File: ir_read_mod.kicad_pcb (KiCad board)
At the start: 2 copper layers, 42 x 42 mm, 25 parts, among them J1 Conn_01x04_Female, J2 Conn_01x05_Female, J3 Conn_01x01_Female, J4 Conn_01x02_Female, Q1 Q_Photo_NPN, SW1 SW_Coded_SH-7070, SW2 SW_SPDT, U1 PIC16F1503-IP

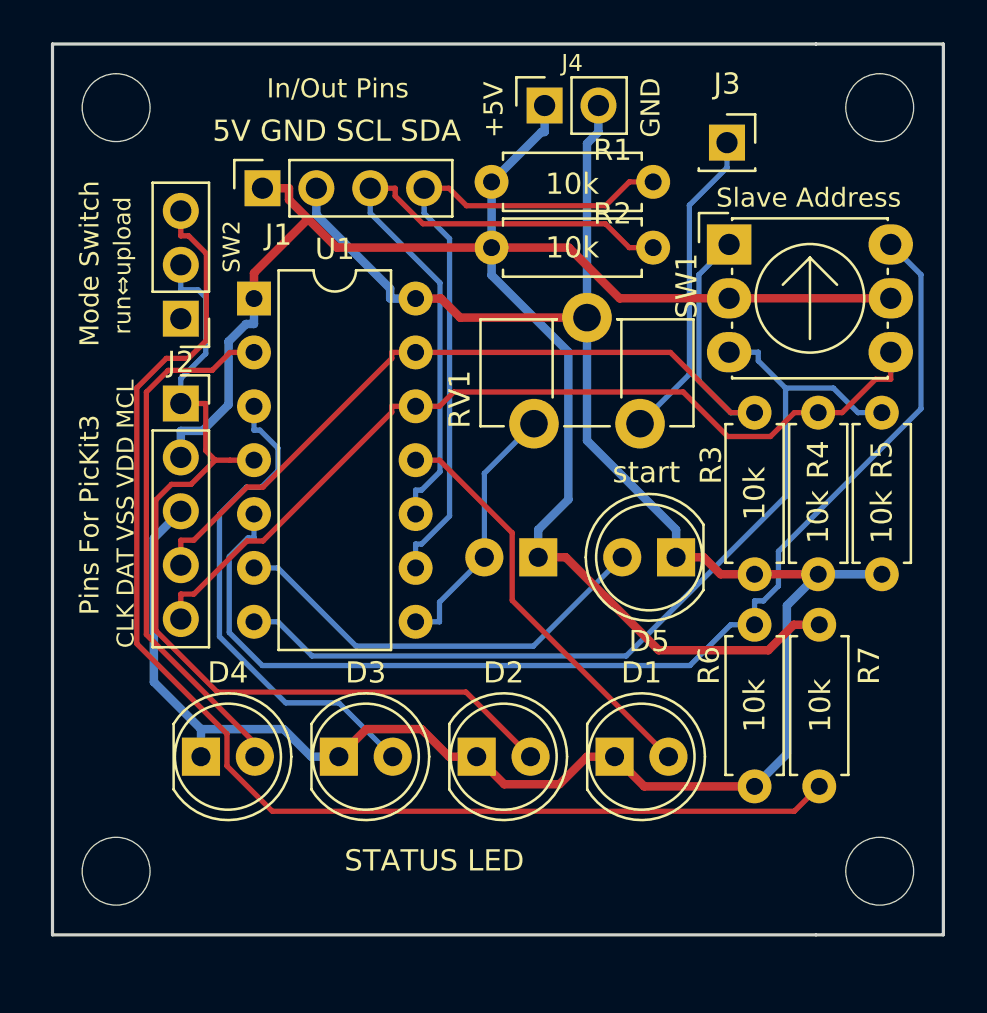
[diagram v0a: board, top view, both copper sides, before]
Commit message: Update: fix parts
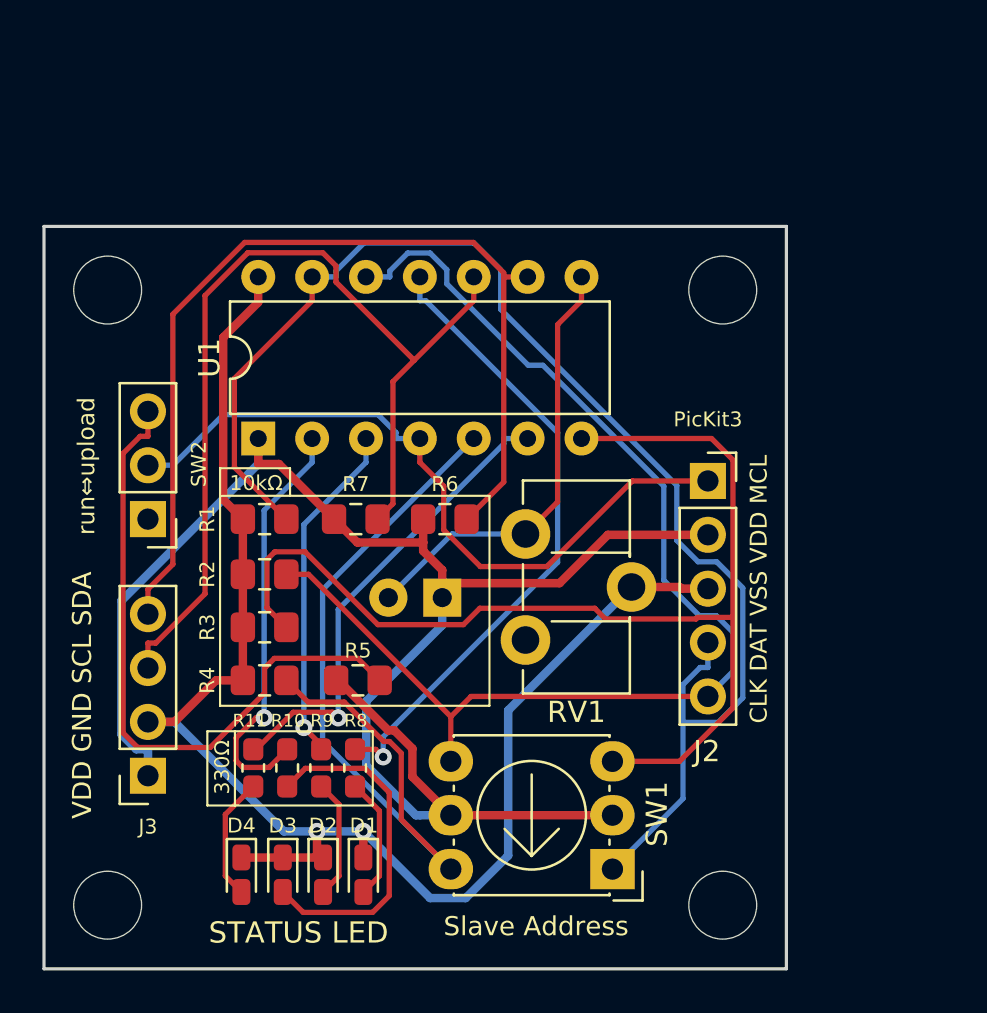
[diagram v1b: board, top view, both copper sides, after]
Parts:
- removed D5: LED, LED_THT:LED_D5.0mm
- removed J1: Conn_01x04_Female, Connector_PinSocket_2.54mm:PinSocket_1x04_P2.54mm_Vertical
- removed J4: Conn_01x02_Female, Connector_PinSocket_2.54mm:PinSocket_1x02_P2.54mm_Vertical
- added R10: 300, Resistor_SMD:R_0603_1608Metric_Pad1.05x0.95mm_HandSolder, F.Cu at (47.5, 69.5)
- added R11: 300, Resistor_SMD:R_0603_1608Metric_Pad1.05x0.95mm_HandSolder, F.Cu at (45.9, 69.5)
- added R8: 300, Resistor_SMD:R_0603_1608Metric_Pad1.05x0.95mm_HandSolder, F.Cu at (50.7, 69.5)
- added R9: 300, Resistor_SMD:R_0603_1608Metric_Pad1.05x0.95mm_HandSolder, F.Cu at (49.1, 69.5)
- D1, D2, D3, D4: footprint LED_THT:LED_D5.0mm -> LED_SMD:LED_0603_1608Metric_Castellated
- J3: value Conn_01x01_Female -> Conn_01x04_Female; footprint Connector_PinSocket_2.54mm:PinSocket_1x01_P2.54mm_Vertical -> Connector_PinSocket_2.54mm:PinSocket_1x04_P2.54mm_Vertical
- R1, R2, R3, R4, R5, R6, R7: footprint Resistor_THT:R_Axial_DIN0207_L6.3mm_D2.5mm_P7.62mm_Horizontal -> Resistor_SMD:R_0805_2012Metric_Pad1.15x1.40mm_HandSolder
- moved J3 40.5 mm to (40.9, 69.9), turned to 180 degrees
- moved SW1 30.0 mm to (62.8, 74.3), turned to 180 degrees
- moved R4 26.6 mm to (46.4, 65.4), turned to 0 degrees
- moved R7 25.2 mm to (50.7, 57.8), turned to 0 degrees
- moved R5 25.2 mm to (50.8, 65.4), turned to 180 degrees
- moved J2 25.1 mm to (67.3, 56.0)
- moved R3 23.2 mm to (46.4, 62.9), turned to 0 degrees
- moved R6 19.3 mm to (54.9, 57.8), turned to 0 degrees
- moved R1 19.2 mm to (46.4, 57.8)
- moved R2 18.8 mm to (46.4, 60.4)
- moved D1 13.1 mm to (51.1, 74.6), turned to 270 degrees
- moved hole2 11.3 mm to (68.0, 47.0)
- moved SW2 9.58 mm to (40.9, 57.8)
- moved D2 9.14 mm to (49.2, 74.6), turned to 270 degrees
- moved hole1 8.61 mm to (39.0, 47.0)
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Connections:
- J2 pad 1: Net-(D2-Pad2) -> Net-(J2-Pad1)
- J3 pad 1: Net-(J3-Pad1) -> +5V
- R1 pad 1: +5V -> GND
- R1 pad 2: Net-(J1-Pad4) -> Net-(J2-Pad4)
- R2 pad 1: +5V -> GND
- R2 pad 2: Net-(J1-Pad3) -> Net-(J2-Pad5)
- R3 pad 2: Net-(J2-Pad4) -> RC3
- R4 pad 2: Net-(J2-Pad5) -> RC5
- R5 pad 1: GND -> Net-(R5-Pad1)
- R5 pad 2: RC3 -> +5V
- R6 pad 1: GND -> +5V
- R6 pad 2: RC5 -> Net-(J3-Pad4)
- R7 pad 1: Net-(R7-Pad1) -> +5V
- R7 pad 2: +5V -> Net-(J3-Pad3)
- RV1 pad 3: Net-(J3-Pad1) -> (no net)
- SW2 pad 1: Net-(SW2-Pad1) -> (no net)
- SW2 pad 2: Net-(D2-Pad2) -> Net-(J2-Pad1)
- SW2 pad 3: Net-(R7-Pad1) -> Net-(R5-Pad1)
- U1 pad 10: Net-(J1-Pad3) -> Net-(J3-Pad3)
- U1 pad 11: Net-(D1-Pad2) -> Net-(R8-Pad1)
- U1 pad 2: Net-(D4-Pad2) -> Net-(R10-Pad1)
- U1 pad 3: Net-(D3-Pad2) -> Net-(R9-Pad1)
- U1 pad 4: Net-(D2-Pad2) -> Net-(J2-Pad1)
- U1 pad 9: Net-(J1-Pad4) -> Net-(J3-Pad4)
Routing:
- net Net-(R7-Pad1): track 59.9 -> 0.00 mm
- net Net-(J3-Pad4): track 0.00 -> 45.7 mm
- net Net-(J3-Pad3): track 0.00 -> 45.4 mm
- net Net-(D2-Pad2): track 43.7 -> 5.63 mm
- net Net-(J2-Pad1): track 0.00 -> 34.1 mm
- net Net-(J1-Pad3): track 32.1 -> 0.00 mm
- net GND: track 103.2 -> 71.7 mm, vias 0 -> 2
- net Net-(R5-Pad1): track 0.00 -> 31.1 mm
- net Net-(J1-Pad4): track 30.8 -> 0.00 mm
- net Net-(R8-Pad1): track 0.00 -> 30.4 mm, vias 0 -> 1
- net Net-(J2-Pad4): track 43.5 -> 65.7 mm
- net Net-(R10-Pad1): track 0.00 -> 19.8 mm, vias 0 -> 1
- net Net-(D4-Pad2): track 25.2 -> 5.83 mm
- net Net-(R9-Pad1): track 0.00 -> 16.2 mm, vias 0 -> 1
- net RC5: track 54.5 -> 39.0 mm
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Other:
- board size 42 x 42 mm -> 35 x 35 mm
- board text added: "10kΩ"
- board text added: "330Ω"
- board text added: "Lchika"
- board text added: "PicKit3"
- board text added: "VDD GND SCL SDA"
- board text added: "ir_recv_board v2.0"
- board text removed: "+5V"
- board text removed: "5V GND SCL SDA"
- board text removed: "GND"
- board text removed: "In/Out Pins"
- board text removed: "Mode Switch"
- board text removed: "Pins For PicKit3"
- board text removed: "ir_recv_board v1.1"
- board text removed: "start"
